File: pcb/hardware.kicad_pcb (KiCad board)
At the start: 4 copper layers, 166 parts, among them J1 Micro_SD_Card_Det_Hirose_DM3AT, J2 USB_A, J3 USB_A, U1 AS4C512M16D3L-12BIN, U2 A33, U3 TPS62095RGTR, U4 TPS62095RGTR, U5 TPS62095RGTR, U6 TPS62095RGTR, U7 AP131-25, U8 MPM-15-5, Y1 24Mhz, Y2 32.768khz

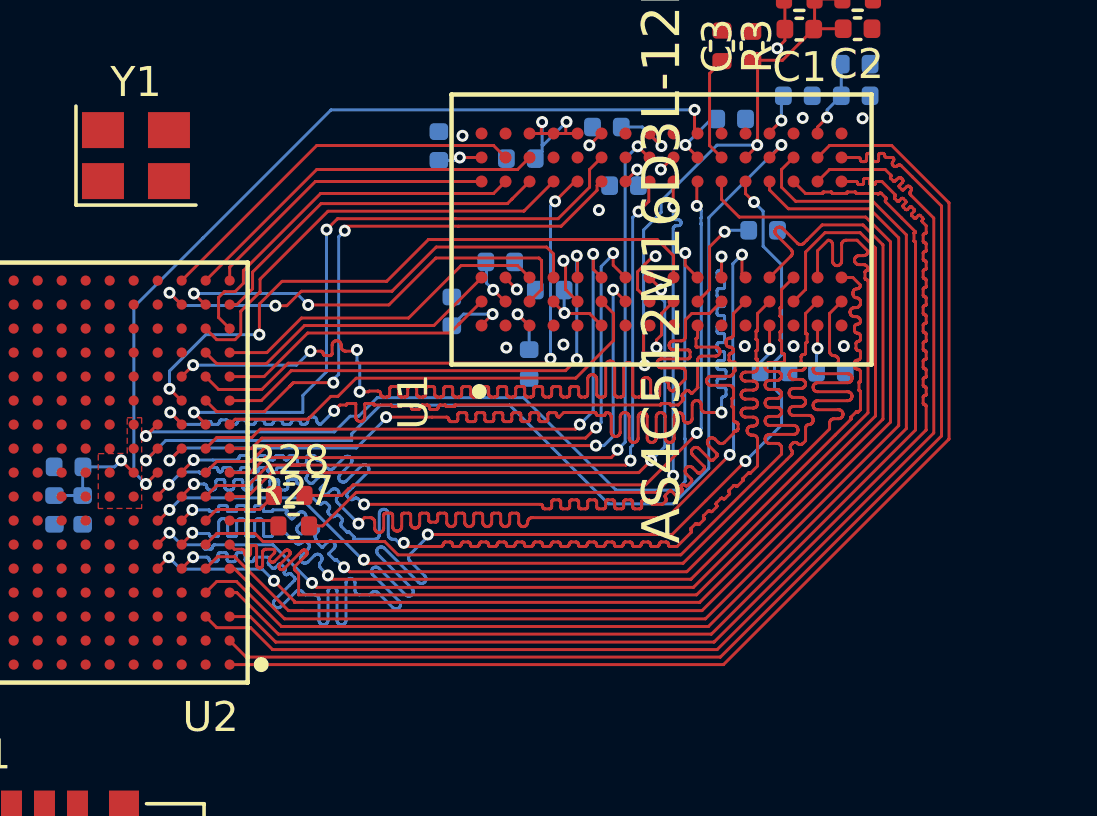
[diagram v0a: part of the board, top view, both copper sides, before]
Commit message: Unsaved changes.
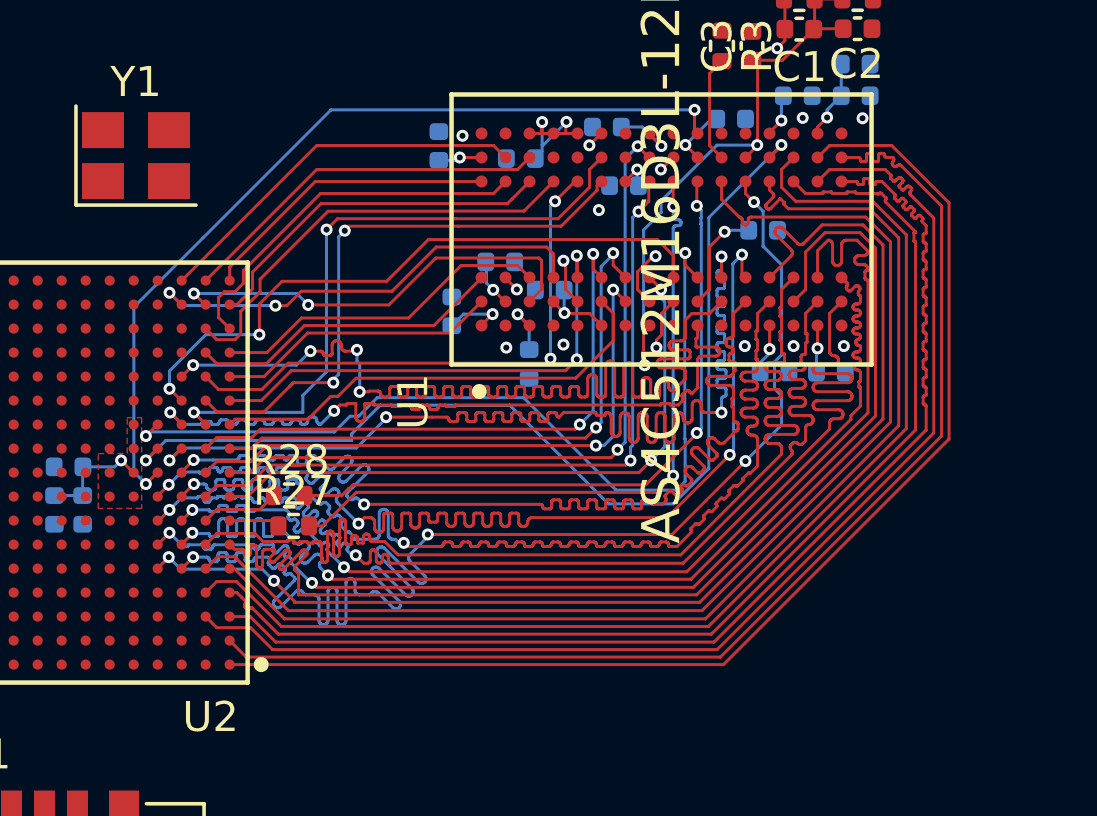
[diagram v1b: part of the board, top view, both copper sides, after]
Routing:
- net adr2: track 32.7 -> 38.0 mm
- net adr7: track 32.8 -> 37.3 mm
- net /ram/!RST: track 39.1 -> 37.4 mm
- net adr9: track 37.8 -> 39.1 mm
- net adr12: track 37.2 -> 38.1 mm
- net adr13: track 37.4 -> 38.0 mm
